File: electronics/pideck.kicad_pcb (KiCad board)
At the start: 2 copper layers, 35 parts, among them J1 Conn_01x20_Socket, J2 Conn_01x20_Socket, J3 BM20B_0.8_-34DS-0.4V_53_, Q1 RE1C002UNTCL, Q2 RE1C002UNTCL, Q3 RE1C002UNTCL, Q4 RE1C002UNTCL, Q5 RE1C002UNTCL, Q6 RE1C002UNTCL, Q7 RE1C002UNTCL, Q8 RE1C002UNTCL

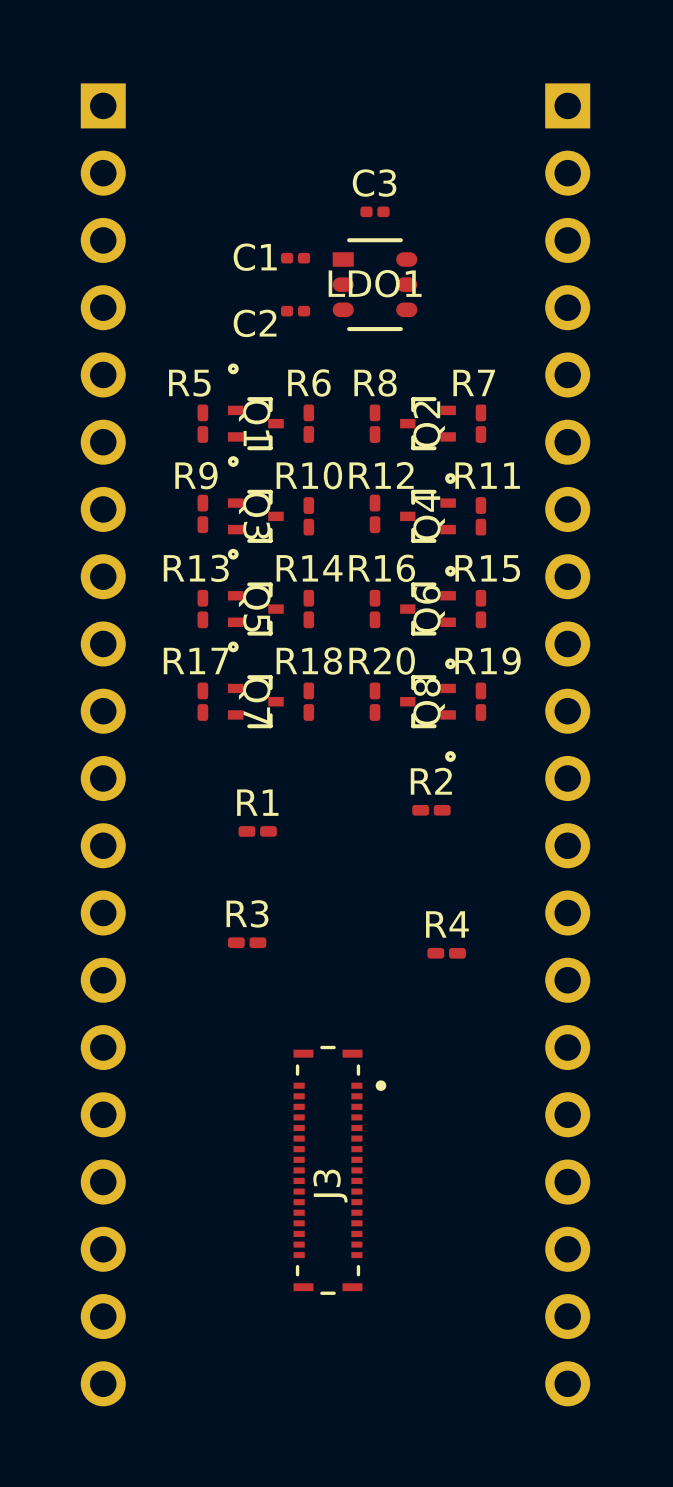
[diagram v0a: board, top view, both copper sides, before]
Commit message: routed
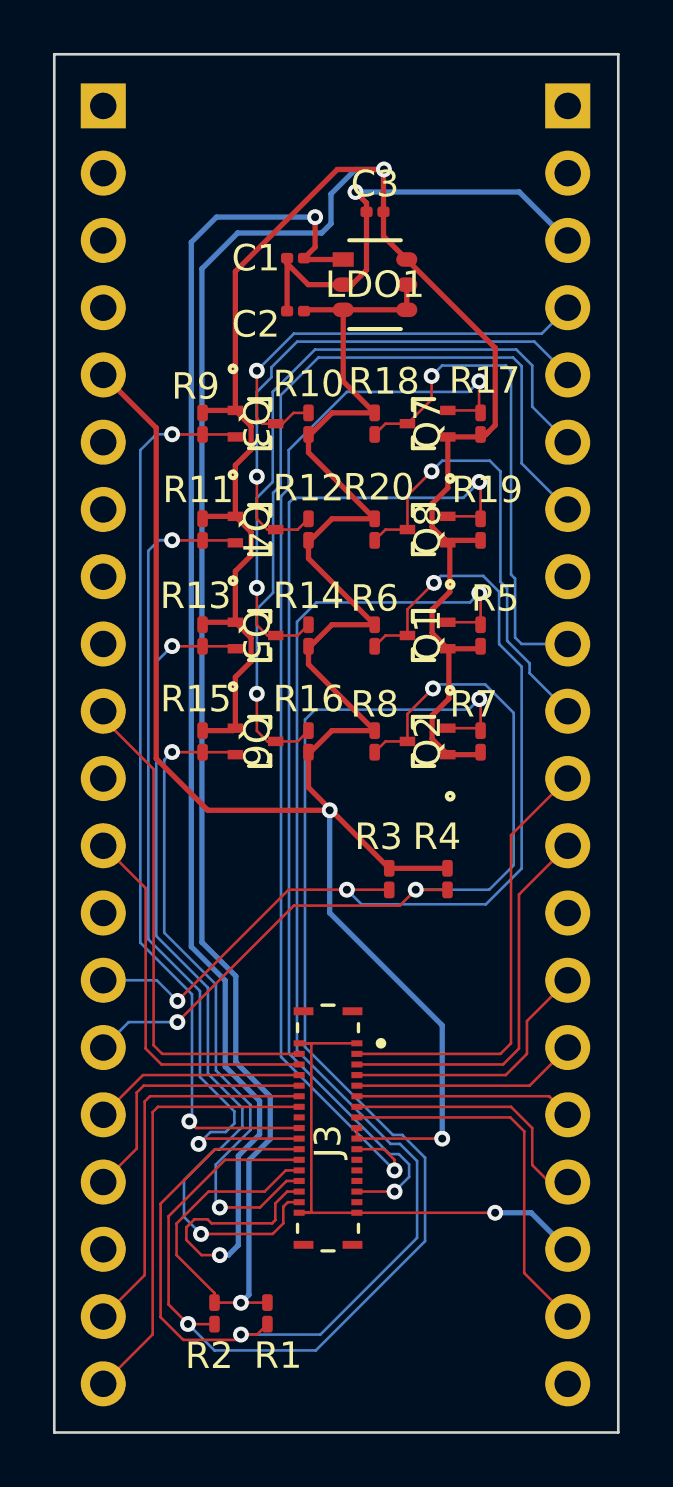
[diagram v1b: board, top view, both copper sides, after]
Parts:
- moved R2 20.7 mm to (104.2, 145.6), turned to 90 degrees
- moved R1 18.2 mm to (106.2, 145.6), turned to 90 degrees
- moved R17 14.8 mm to (114.2, 112.0), turned to 90 degrees
- moved R5 13.2 mm to (114.2, 120.0), turned to 90 degrees
- moved Q7 12.3 mm to (112.2, 112.0), turned to 90 degrees
- moved Q2 12.0 mm to (112.2, 124.0)
- moved R7 12.0 mm to (114.2, 124.0)
- moved R8 12.0 mm to (110.2, 124.0), turned to -90 degrees
- moved R15 11.6 mm to (103.8, 124.0), turned to -90 degrees
- moved R18 10.8 mm to (110.2, 112.0), turned to -90 degrees
- moved R11 10.5 mm to (103.8, 116.0), turned to -90 degrees
- moved Q1 10.3 mm to (112.2, 120.0), turned to 90 degrees
- moved R6 8.38 mm to (110.2, 120.0)
- moved Q6 8.21 mm to (105.8, 124.0), turned to -90 degrees
- moved Q4 6.53 mm to (105.8, 116.0), turned to -90 degrees
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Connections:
- J1 pad 13: GND -> unconnected-(J1-GND-Pad13)
- J1 pad 4: unconnected-(J1-GP2-Pad4) -> TP_MOTION_3V3
- J1 pad 5: unconnected-(J1-GP3-Pad5) -> TP_SHUTDOWN_3V3
- J1 pad 6: unconnected-(J1-GP4-Pad6) -> TP_RESET_3V3
- J1 pad 7: unconnected-(J1-GP5-Pad7) -> TP_BLK_LED_K_3V3
- J1 pad 8: GND -> unconnected-(J1-GND-Pad8)
- J2 pad 13: GND -> unconnected-(J2-GND-Pad13)
- J2 pad 18: GND -> unconnected-(J2-GND-Pad18)
- J2 pad 3: GND -> unconnected-(J2-GND-Pad3)
- J2 pad 8: GND -> unconnected-(J2-GND-Pad8)
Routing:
- net +1V8: track 0.00 -> 122.8 mm, vias 0 -> 2
- net KB_BLK_LED_A: track 0.00 -> 81.2 mm, vias 0 -> 2
- net TP_SCL_1V8: track 0.00 -> 58.2 mm, vias 0 -> 2
- net +2V8: track 0.00 -> 55.6 mm, vias 0 -> 2
- net TP_SDA_1V8: track 0.00 -> 53.3 mm, vias 0 -> 2
- net KB_BLK_LED_K_1V8: track 0.00 -> 41.6 mm, vias 0 -> 2
- net PANNEL_BLK_LED_K_1V8: track 0.00 -> 39.8 mm, vias 0 -> 2
- net GND: track 0.00 -> 37.8 mm, vias 0 -> 2
- net TP_SCL_3V3: track 0.00 -> 37.7 mm, vias 0 -> 3
- net TP_MOTION_1V8: track 0.00 -> 34.2 mm, vias 0 -> 2
- net TP_SDA_3V3: track 0.00 -> 32.7 mm, vias 0 -> 3
- net TP_RESET_1V8: track 0.00 -> 32.0 mm, vias 0 -> 2
- net TP_SHUTDOWN_1V8: track 0.00 -> 31.6 mm, vias 0 -> 2
- net TP_BLK_LED_K_3V3: track 0.00 -> 31.3 mm, vias 0 -> 1
- net TP_RESET_3V3: track 0.00 -> 25.5 mm, vias 0 -> 1
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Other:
- board outline added: 21.3 x 52 mm
